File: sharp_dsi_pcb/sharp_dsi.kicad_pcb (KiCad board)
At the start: 2 copper layers, 1 part

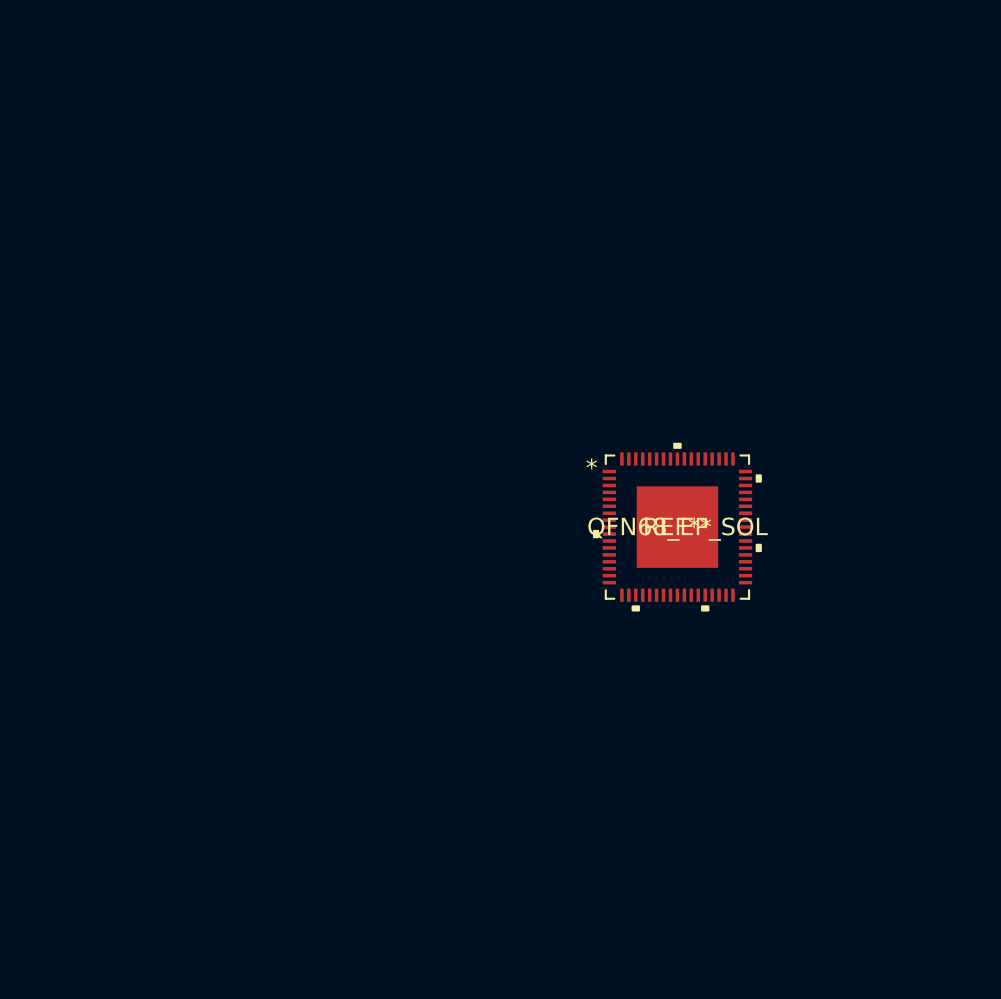
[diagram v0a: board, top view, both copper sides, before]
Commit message: pcb status gbr-v0.2
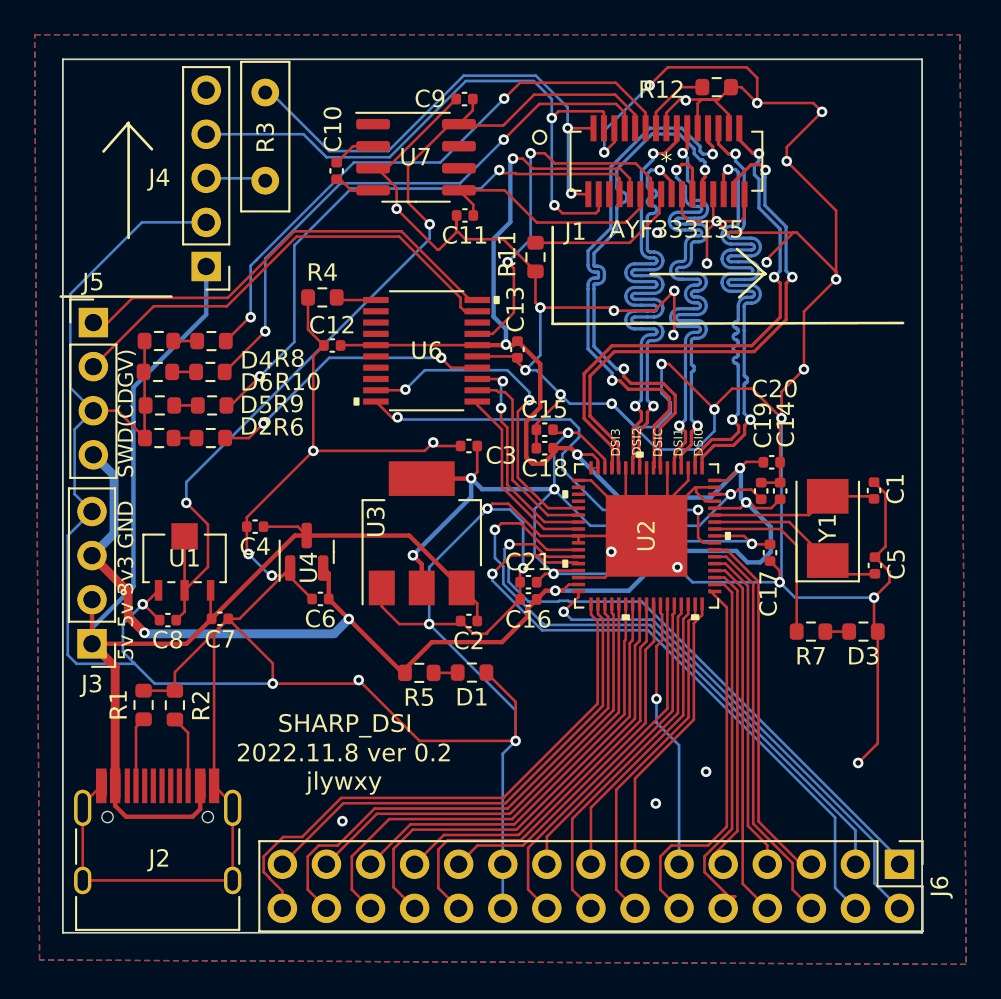
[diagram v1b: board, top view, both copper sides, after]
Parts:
- removed REF**: QFN68_EP_SOL, footprints:SSD2828QN4
- added C1: 10pF, Capacitor_SMD:C_0402_1005Metric, F.Cu at (133.2, 74.1)
- added C10: 100nF, Capacitor_SMD:C_0402_1005Metric, F.Cu at (102.3, 55.7)
- added C11: 100nF, Capacitor_SMD:C_0402_1005Metric, F.Cu at (109.7, 58.2)
- added C12: 100nF, Capacitor_SMD:C_0402_1005Metric, F.Cu at (102.0, 65.7)
- added C13: 100nF, Capacitor_SMD:C_0402_1005Metric, F.Cu at (112.7, 66.0)
- added C14: 100nF, Capacitor_SMD:C_0402_1005Metric, F.Cu at (127.8, 74.1)
- added C15: 100nF, Capacitor_SMD:C_0402_1005Metric, F.Cu at (114.3, 70.6)
- added C16: 100nF, Capacitor_SMD:C_0402_1005Metric, F.Cu at (113.3, 80.4)
- added C17: 100nF, Capacitor_SMD:C_0402_1005Metric, F.Cu at (127.3, 77.7)
- added C18: 100nF, Capacitor_SMD:C_0402_1005Metric, F.Cu at (114.3, 71.7)
- added C19: 100nF, Capacitor_SMD:C_0402_1005Metric, F.Cu at (126.7, 74.1)
- added C2: 100nF, Capacitor_SMD:C_0402_1005Metric, F.Cu at (109.9, 81.6)
- added C20: 100nF, Capacitor_SMD:C_0402_1005Metric, F.Cu at (127.4, 72.5)
- added C21: 100nF, Capacitor_SMD:C_0402_1005Metric, F.Cu at (113.3, 79.4)
- added C3: 100nF, Capacitor_SMD:C_0402_1005Metric, F.Cu at (109.9, 71.5)
- added C4: 100nF, Capacitor_SMD:C_0402_1005Metric, F.Cu at (97.6, 76.2)
- added C5: 10pF, Capacitor_SMD:C_0402_1005Metric, F.Cu at (133.3, 78.4)
- added C6: 100nF, Capacitor_SMD:C_0402_1005Metric, F.Cu at (101.3, 80.3)
- added C7: 100nF, Capacitor_SMD:C_0402_1005Metric, F.Cu at (95.6, 81.5)
- added C8: 100nF, Capacitor_SMD:C_0402_1005Metric, F.Cu at (92.6, 81.6)
- added C9: 100nF, Capacitor_SMD:C_0402_1005Metric, F.Cu at (109.7, 51.5)
- added D1: LED, Resistor_SMD:R_0603_1608Metric, F.Cu at (110.1, 84.6)
- added D2: LED, Resistor_SMD:R_0603_1608Metric, F.Cu at (92.1, 71.1)
- added D3: LED, Resistor_SMD:R_0603_1608Metric, F.Cu at (132.6, 82.2)
- added D4: LED, Resistor_SMD:R_0603_1608Metric, F.Cu at (92.0, 65.5)
- added D5: LED, Resistor_SMD:R_0603_1608Metric, F.Cu at (92.1, 69.2)
- added D6: LED, Resistor_SMD:R_0603_1608Metric, F.Cu at (92.0, 67.3)
- added J1: AYF333135, footprints:AYF333135, F.Cu at (121.3, 55.1)
- added J2: USB_C_Receptacle_USB2.0, Connector_USB:USB_C_Receptacle_HRO_TYPE-C-31-M-12, F.Cu at (92.0, 95.5)
- added J3: Conn_01x04_Male, Connector_PinHeader_2.54mm:PinHeader_1x04_P2.54mm_Vertical, F.Cu at (88.2, 82.9)
- added J4: Conn_01x05, Connector_PinHeader_2.54mm:PinHeader_1x05_P2.54mm_Vertical, F.Cu at (94.8, 61.2)
- added J5: Conn_01x04_Male, Connector_PinHeader_2.54mm:PinHeader_1x04_P2.54mm_Vertical, F.Cu at (88.3, 64.4)
- added J6: Conn_02x15_Counter_Clockwise, Connector_PinHeader_2.54mm:PinHeader_2x15_P2.54mm_Vertical, F.Cu at (134.7, 95.6)
- added R1: 5.1k, Resistor_SMD:R_0603_1608Metric, F.Cu at (91.2, 86.4)
- added R10: 5.6k, Resistor_SMD:R_0603_1608Metric, F.Cu at (95.0, 67.3)
- added R11: 100k, Resistor_SMD:R_0603_1608Metric, F.Cu at (113.7, 60.6)
- added R12: 100k, Resistor_SMD:R_0603_1608Metric, F.Cu at (124.2, 50.9)
- added R2: 5.1k, Resistor_SMD:R_0603_1608Metric, F.Cu at (93.0, 86.5)
- added R3: 220, Resistor_THT:R_Box_L8.4mm_W2.5mm_P5.08mm, F.Cu at (98.2, 51.2)
- added R4: 10k, Resistor_SMD:R_0603_1608Metric, F.Cu at (101.5, 63.0)
- added R5: 5.6k, Resistor_SMD:R_0603_1608Metric, F.Cu at (107.0, 84.6)
- added R6: 5.6k, Resistor_SMD:R_0603_1608Metric, F.Cu at (95.0, 71.1)
- added R7: 5.6k, Resistor_SMD:R_0603_1608Metric, F.Cu at (129.6, 82.2)
- added R8: 5.6k, Resistor_SMD:R_0603_1608Metric, F.Cu at (95.1, 65.5)
- added R9: 5.6k, Resistor_SMD:R_0603_1608Metric, F.Cu at (95.1, 69.2)
- added U1: XC6206PxxxMR, footprints:XC6206P502PR, F.Cu at (93.5, 78.0)
- added U2: SSD2828QN4, footprints:SSD2828QN4, F.Cu at (120.1, 76.7)
- added U3: AMS1117, Package_TO_SOT_SMD:SOT-223-3_TabPin2, F.Cu at (107.2, 76.6)
- added U4: XC6206PxxxMR, Package_TO_SOT_SMD:SOT-23, F.Cu at (100.6, 77.6)
- added U6: STM32F030F4Px, footprints:STM32F030F4P6, F.Cu at (107.5, 66.0)
- added U7: ICL7660, Package_SO:SOIC-8_3.9x4.9mm_P1.27mm, F.Cu at (106.9, 54.9)
- added Y1: Crystal, Crystal:Crystal_SMD_5032-2Pin_5.0x3.2mm, F.Cu at (130.6, 76.3)
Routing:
- net GND: track 0.00 -> 444.0 mm, vias 0 -> 42
- net /SSD_PS0: track 0.00 -> 126.9 mm, vias 0 -> 8
- net /5v: track 0.00 -> 75.3 mm
- net /SSD_MVDD: track 0.00 -> 64.6 mm, vias 0 -> 7
- net /LCD_AVDD+: track 0.00 -> 54.8 mm, vias 0 -> 2
- net /SSD_RGB_PCLK: track 0.00 -> 37.1 mm, vias 0 -> 1
- net /SSD_RGB_DEN: track 0.00 -> 37.0 mm, vias 0 -> 1
- net /LCD_BL_GND: track 0.00 -> 36.7 mm, vias 0 -> 2
- net /SSD_RGB_HSYNC: track 0.00 -> 36.1 mm, vias 0 -> 1
- net /LCD_OUT_BLPWM: track 0.00 -> 33.7 mm, vias 0 -> 2
- net /LCD_OUT_HSYNC: track 0.00 -> 33.0 mm, vias 0 -> 2
- net /LCD_OUT_TE: track 0.00 -> 32.6 mm, vias 0 -> 2
- net /SSD_RGB_R0: track 0.00 -> 32.2 mm
- net /LCD_DSI_D3N: track 0.00 -> 31.6 mm, vias 0 -> 2
- net /LCD_DSI_CLKN: track 0.00 -> 31.6 mm, vias 0 -> 2
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- added copper zone on B.Cu, net GND
- added copper zone on F.Cu, net GND
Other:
- board outline added: 49.5 x 50.3 mm
- board text added: "2022.11.8 ver 0.2 jlywxy"
- board text added: "5v 5v 3v3 GND"
- board text added: "DSI0"
- board text added: "DSI1"
- board text added: "DSI2"
- board text added: "DSI3"
- board text added: "DSIC"
- board text added: "SHARP_DSI"
- board text added: "SWD(CDGV)"
